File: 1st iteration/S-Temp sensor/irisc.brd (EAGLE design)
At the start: 22.8 x 45.4 mm, 11 parts, among them U6 ANALOG_DEVICES_AD7997BRUZ-1RE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

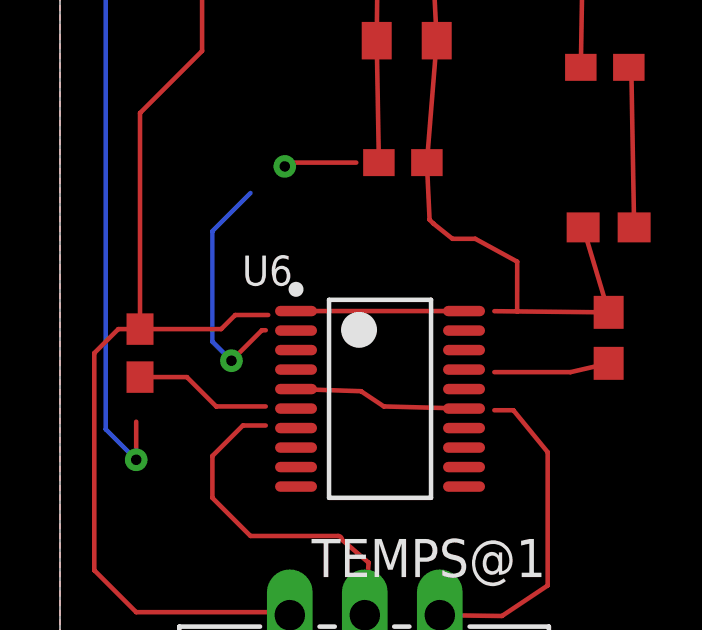
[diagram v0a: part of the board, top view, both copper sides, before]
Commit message: Sabina Changes
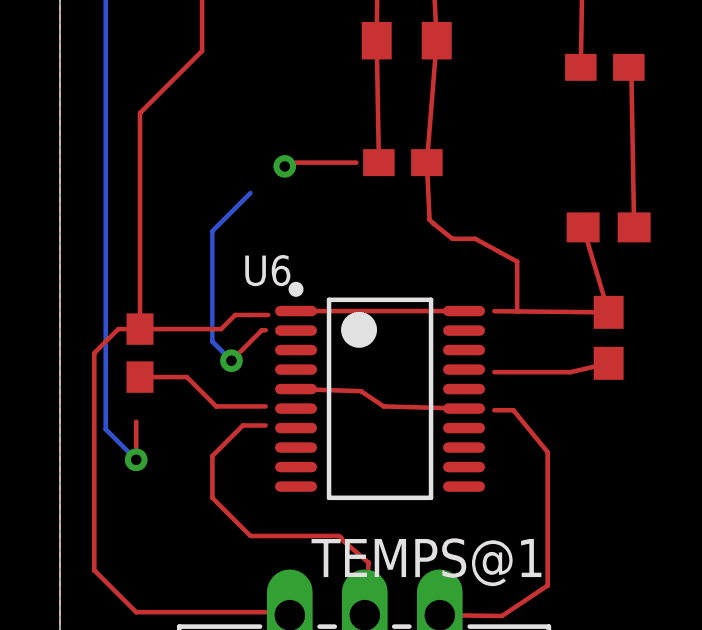
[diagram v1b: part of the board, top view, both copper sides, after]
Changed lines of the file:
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@@
 <wire x1="2.667" y1="24.676" x2="5.372" y2="24.676" width="0.1524" layer="1"/>
 <wire x1="5.372" y1="24.676" x2="5.842" y2="25.146" width="0.1524" layer="1"/>
-<wire x1="5.842" y1="25.146" x2="6.9418" y2="25.146" width="0.1524" layer="1"/>
+<wire x1="5.842" y1="25.146" x2="6.35" y2="25.146" width="0.1524" layer="1"/>
+<wire x1="6.35" y1="25.146" x2="6.9418" y2="25.146" width="0.1524" layer="1"/>
 <wire x1="2.667" y1="24.676" x2="2.667" y2="31.877" width="0.1524" layer="1"/>
 <wire x1="4.737" y1="33.947" x2="4.737" y2="40.894" width="0.1524" layer="1"/>
